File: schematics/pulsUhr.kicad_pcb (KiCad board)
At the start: 2 copper layers, 59.7 x 24.1 mm, 17 parts, among them IC1 APDS-9006-020, P1 CONN_01X04, Q1 ZVN2106G, U1 MCP6002

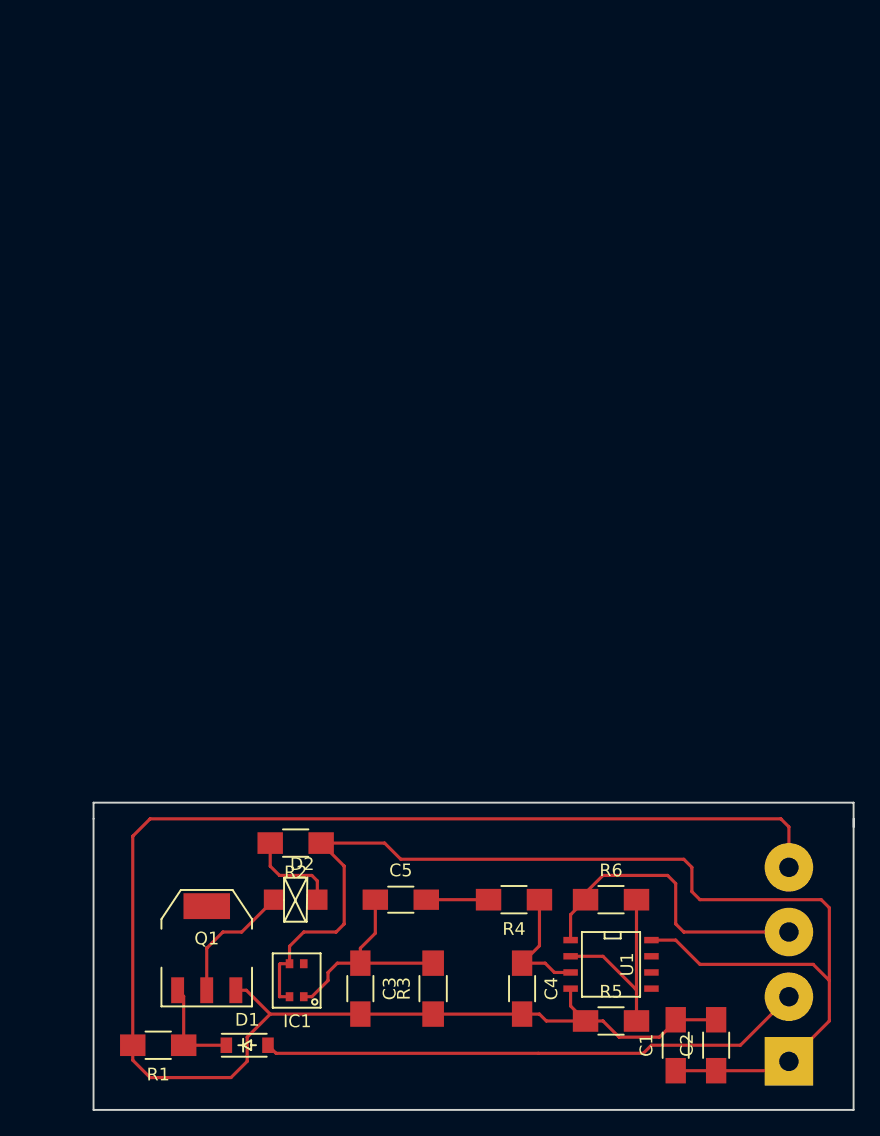
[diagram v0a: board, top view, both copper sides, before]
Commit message: New Layout for version 0.1
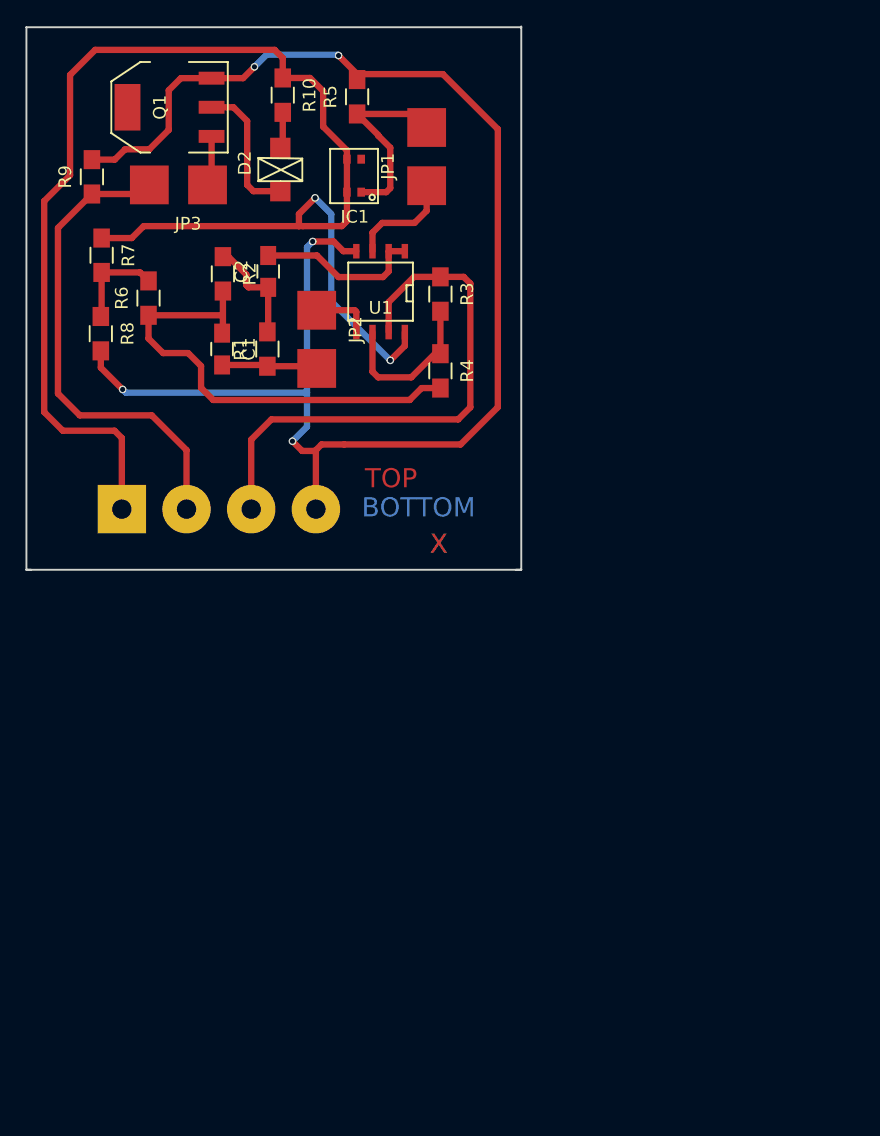
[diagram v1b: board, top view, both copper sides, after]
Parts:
- removed C3: 10µF, Capacitors_SMD:C_1206_HandSoldering
- removed C4: 3,3nF, Capacitors_SMD:C_1206_HandSoldering
- removed C5: 100nF, Capacitors_SMD:C_1206_HandSoldering
- removed D1: D, Diodes_SMD:SOD-123
- added JP1: Jumper_NC_Small, SemesterProjekt:SOLDER_JUMPER, F.Cu at (138.6, 34.6)
- added JP2: Jumper_NC_Small, SemesterProjekt:SOLDER_JUMPER, F.Cu at (129.9, 53.5)
- added JP3: Jumper_NC_Small, SemesterProjekt:SOLDER_JUMPER, F.Cu at (116.8, 39.1)
- added R10: 150, Resistors_SMD:R_0805_HandSoldering, F.Cu at (127.3, 32.1)
- added R7: 10K, Resistors_SMD:R_0805_HandSoldering, F.Cu at (113.0, 44.6)
- added R8: 10K, Resistors_SMD:R_0805_HandSoldering, F.Cu at (113.0, 50.8)
- added R9: 100k, Resistors_SMD:R_0805_HandSoldering, F.Cu at (112.3, 38.5)
- C1: value C -> 82nF; footprint Capacitors_SMD:C_1206_HandSoldering -> Capacitors_SMD:C_0805_HandSoldering
- C2: value C -> 3,3nF; footprint Capacitors_SMD:C_1206_HandSoldering -> Capacitors_SMD:C_0805_HandSoldering
- R1: value 100k -> 10M; footprint Resistors_SMD:R_1206_HandSoldering -> Resistors_SMD:R_0805_HandSoldering
- R2: value 150 -> 10M; footprint Resistors_SMD:R_1206_HandSoldering -> Resistors_SMD:R_0805_HandSoldering
- R3: value 1k -> 2K8; footprint Resistors_SMD:R_1206_HandSoldering -> Resistors_SMD:R_0805_HandSoldering
- R4: value 10M -> 200; footprint Resistors_SMD:R_1206_HandSoldering -> Resistors_SMD:R_0805_HandSoldering
- R5: value 200 -> 1K; footprint Resistors_SMD:R_1206_HandSoldering -> Resistors_SMD:R_0805_HandSoldering
- R6: value 2k8 -> 100K; footprint Resistors_SMD:R_1206_HandSoldering -> Resistors_SMD:R_0805_HandSoldering
- moved R5 75.3 mm to (133.1, 32.2), turned to 90 degrees
- moved C2 70.2 mm to (126.1, 45.9)
- moved Q1 66.1 mm to (118.4, 33.0), turned to 90 degrees
- moved C1 65.3 mm to (122.5, 52.0), turned to 270 degrees
- moved IC1 63.3 mm to (133.4, 39.7)
- moved R6 59.6 mm to (116.7, 48.0), turned to 90 degrees
- moved D2 57.4 mm to (127.1, 37.9), turned to 90 degrees
- moved P1 57.3 mm to (122.2, 64.6), turned to 0 degrees
- moved U1 55.8 mm to (134.9, 47.5), turned to 180 degrees
- moved R1 55.3 mm to (126.0, 52.0), turned to 90 degrees
- moved R3 54.5 mm to (139.6, 47.7), turned to 270 degrees
- moved R2 45.1 mm to (122.6, 46.1), turned to 270 degrees
- moved R4 41.9 mm to (139.6, 53.7), turned to 270 degrees
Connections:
- C1 pad 1: +5V -> VGND
- C1 pad 2: GND -> Net-(C1-Pad2)
- C2 pad 1: +5V -> Net-(C2-Pad1)
- C2 pad 2: GND -> Net-(C2-Pad2)
- IC1 pad 1: Net-(C3-Pad1) -> Net-(IC1-Pad1)
- Q1 pad 1: Net-(D1-Pad1) -> Net-(JP3-Pad2)
- R1 pad 1: Net-(D1-Pad1) -> Net-(C1-Pad2)
- R1 pad 2: GND -> Net-(C2-Pad1)
- R2 pad 1: +5V -> Net-(C2-Pad1)
- R2 pad 2: Net-(D2-Pad2) -> VGND
- R3 pad 1: GND -> OUT
- R3 pad 2: Net-(C3-Pad1) -> Net-(R3-Pad2)
- R4 pad 1: Net-(C4-Pad1) -> Net-(R3-Pad2)
- R4 pad 2: Net-(C5-Pad2) -> VGND
- R5 pad 1: GND -> Net-(IC1-Pad1)
- R5 pad 2: Net-(R5-Pad2) -> GND
- R6 pad 1: OUT -> VGND
- R6 pad 2: Net-(R5-Pad2) -> Net-(R6-Pad2)
- U1 pad 1: OUT -> Net-(C2-Pad2)
- U1 pad 2: Net-(R5-Pad2) -> Net-(C2-Pad2)
- U1 pad 3: Net-(C4-Pad1) -> Net-(JP1-Pad2)
- U1 pad 5: (no net) -> Net-(JP2-Pad2)
- U1 pad 6: (no net) -> Net-(R3-Pad2)
- U1 pad 7: (no net) -> OUT
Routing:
- net VGND: track 0.00 -> 37.4 mm
- net OUT: track 24.4 -> 43.2 mm
- net Net-(C3-Pad1): track 17.1 -> 0.00 mm
- net Net-(R5-Pad2): track 15.9 -> 0.00 mm
- net +5V: track 98.6 -> 114.2 mm, vias 0 -> 2
- net Net-(IC1-Pad1): track 0.00 -> 15.2 mm
- net Net-(R3-Pad2): track 0.00 -> 13.4 mm
- net Net-(C2-Pad2): track 0.00 -> 13.2 mm
- net Net-(C4-Pad1): track 9.66 -> 0.00 mm
- net Net-(C2-Pad1): track 0.00 -> 8.65 mm
- net Net-(JP1-Pad2): track 0.00 -> 8.39 mm
- net GND: track 130.6 -> 122.3 mm, vias 0 -> 5
- net Net-(D1-Pad1): track 7.87 -> 0.00 mm
- net Net-(C1-Pad2): track 0.00 -> 7.68 mm
- net Net-(R6-Pad2): track 0.00 -> 7.44 mm
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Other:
- board size 59.7 x 24.1 mm -> 38.9 x 42.7 mm
- net class Default: trace_width 0.25 -> 0.5
- board text added: "BOTTOM"
- board text added: "TOP"
- board text added: "X"
